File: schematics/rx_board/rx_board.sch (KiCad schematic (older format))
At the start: 15 parts, among them U1 SI4463-C2A-GM, X2 SMA

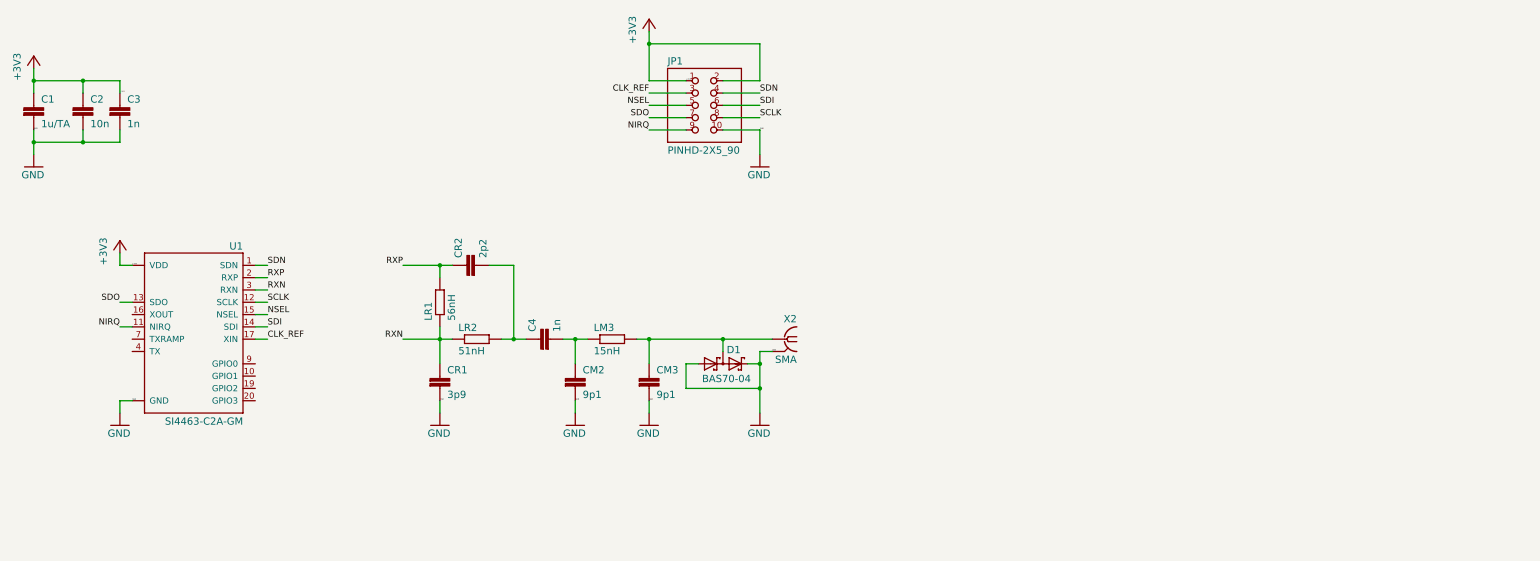
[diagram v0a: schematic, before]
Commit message: first complete design & routing
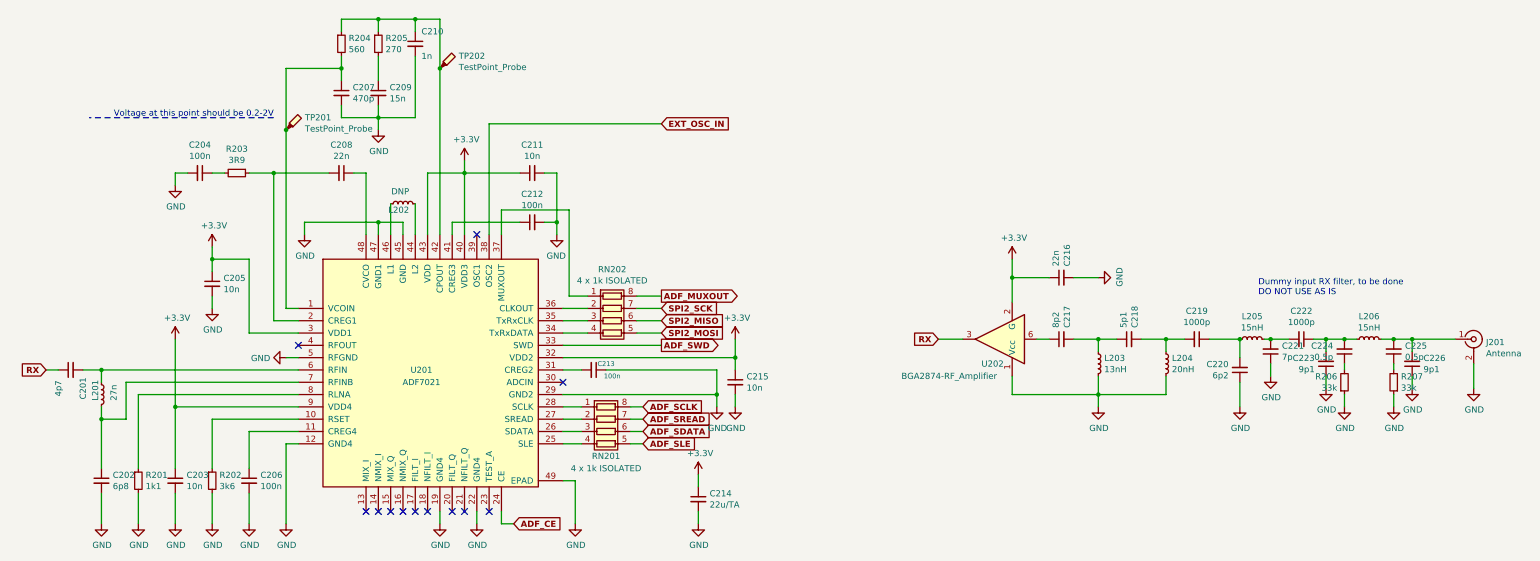
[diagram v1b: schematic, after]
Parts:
- removed C1: 1u/TA, rx_board:C1206, symbol rx_board-eagle-import:C-EUC1206
- removed C2: 10n, rx_board:C0805, symbol rx_board-eagle-import:C-EUC0805
- removed C3, C4: 1n, rx_board:C0805, symbol rx_board-eagle-import:C-EUC0805
- removed CM2, CM3: 9p1, rx_board:C0805, symbol rx_board-eagle-import:C-EUC0805
- removed CR1: 3p9, rx_board:C0805, symbol rx_board-eagle-import:C-EUC0805
- removed CR2: 2p2, rx_board:C0805, symbol rx_board-eagle-import:C-EUC0805
- removed D1: BAS70-04, rx_board:SOT23, symbol rx_board-eagle-import:BAS70-04
- removed JP1: PINHD-2X5_90, rx_board:2X05_90, symbol rx_board-eagle-import:PINHD-2X5_90
- removed LM3: 15nH, rx_board:R0805, symbol rx_board-eagle-import:R-EU_R0805
- removed LR1: 56nH, rx_board:R0805, symbol rx_board-eagle-import:R-EU_R0805
- removed LR2: 51nH, rx_board:R0805, symbol rx_board-eagle-import:R-EU_R0805
- removed U1: SI4463-C2A-GM, rx_board:QFN50P400X400X90-20N, symbol rx_board-eagle-import:SI4463-C2A-GM
- removed X2: SMA, rx_board:J502-ND-142-0701-871_876, symbol rx_board-eagle-import:SMA-142-0701-871_876
- added C201: 4p7, Capacitor_SMD:C_0603_1608Metric, symbol rx_board-rescue:C_Small-Device-Mainboard-rescue-rx_board-rescue
- added C202: 6p8, Capacitor_SMD:C_0603_1608Metric, symbol rx_board-rescue:C_Small-Device-Mainboard-rescue-rx_board-rescue
- added C203, C205, C211, C215: 10n, Capacitor_SMD:C_0603_1608Metric, symbol rx_board-rescue:C_Small-Device-Mainboard-rescue-rx_board-rescue
- added C204, C206, C212, C213: 100n, Capacitor_SMD:C_0603_1608Metric, symbol rx_board-rescue:C_Small-Device-Mainboard-rescue-rx_board-rescue
- added C207: 470p, Capacitor_SMD:C_0603_1608Metric, symbol rx_board-rescue:C_Small-Device-Mainboard-rescue-rx_board-rescue
- added C208, C216: 22n, Capacitor_SMD:C_0603_1608Metric, symbol rx_board-rescue:C_Small-Device-Mainboard-rescue-rx_board-rescue
- added C209: 15n, Capacitor_SMD:C_0603_1608Metric, symbol rx_board-rescue:C_Small-Device-Mainboard-rescue-rx_board-rescue
- added C210: 1n, Capacitor_SMD:C_0603_1608Metric, symbol rx_board-rescue:C_Small-Device-Mainboard-rescue-rx_board-rescue
- added C214: 22u/TA, Capacitor_Tantalum_SMD:CP_EIA-3216-18_Kemet-A, symbol rx_board-rescue:C_Small-device-Mainboard-rescue-rx_board-rescue
- added C217: 8p2, Capacitor_SMD:C_0603_1608Metric, symbol rx_board-rescue:C_Small-Device-Mainboard-rescue-rx_board-rescue
- added C218: 5p1, Capacitor_SMD:C_0603_1608Metric, symbol rx_board-rescue:C_Small-Device-Mainboard-rescue-rx_board-rescue
- added C219, C222: 1000p, Capacitor_SMD:C_0603_1608Metric, symbol rx_board-rescue:C_Small-device-Mainboard-rescue-rx_board-rescue
- added C220: 6p2, Capacitor_SMD:C_0603_1608Metric, symbol rx_board-rescue:C_Small-Device-Mainboard-rescue-rx_board-rescue
- added C221: 7p, Capacitor_SMD:C_0603_1608Metric, symbol rx_board-rescue:C_Small-Device-Mainboard-rescue-rx_board-rescue
- added C223, C226: 9p1, Capacitor_SMD:C_0603_1608Metric, symbol rx_board-rescue:C_Small-device-Mainboard-rescue-rx_board-rescue
- added C224, C225: 0.5p, Capacitor_SMD:C_0603_1608Metric, symbol rx_board-rescue:C_Small-Device-Mainboard-rescue-rx_board-rescue
- added J201: Antenna, Connector_Coaxial:SMA_Samtec_SMA-J-P-X-ST-EM1_EdgeMount, symbol rx_board-rescue:Conn_Coaxial-conn-Mainboard-rescue-rx_board-rescue
- added L201: 27n, Inductor_SMD:L_0603_1608Metric, symbol rx_board-rescue:L_Small-Device-Mainboard-rescue-rx_board-rescue
- added L202: DNP, Inductor_SMD:L_0603_1608Metric, symbol rx_board-rescue:L_Small-Device-Mainboard-rescue-rx_board-rescue
- added L203: 13nH, Inductor_SMD:L_0603_1608Metric, symbol Device:L_Small
- added L204: 20nH, Inductor_SMD:L_0603_1608Metric, symbol Device:L_Small
- added L205: 15nH, Inductor_SMD:L_0603_1608Metric, symbol rx_board-rescue:L_Small-Device-Mainboard-rescue-rx_board-rescue
- added L206: 15nH, Inductor_SMD:L_0603_1608Metric, symbol rx_board-rescue:L_Small-device-Mainboard-rescue-rx_board-rescue
- added R201: 1k1, Resistor_SMD:R_0603_1608Metric, symbol rx_board-rescue:R_Small-Device-Mainboard-rescue-rx_board-rescue
- added R202: 3k6, Resistor_SMD:R_0603_1608Metric, symbol rx_board-rescue:R_Small-Device-Mainboard-rescue-rx_board-rescue
- added R203: 3R9, Resistor_SMD:R_0603_1608Metric, symbol rx_board-rescue:R_Small-Device-Mainboard-rescue-rx_board-rescue
- added R204: 560, Resistor_SMD:R_0603_1608Metric, symbol rx_board-rescue:R_Small-Device-Mainboard-rescue-rx_board-rescue
- added R205: 270, Resistor_SMD:R_0603_1608Metric, symbol rx_board-rescue:R_Small-Device-Mainboard-rescue-rx_board-rescue
- added R206, R207: 33k, Resistor_SMD:R_0603_1608Metric, symbol rx_board-rescue:R_Small-Device-Mainboard-rescue-rx_board-rescue
- added RN201, RN202: 4 x 1k ISOLATED, Resistor_SMD:R_Array_Concave_4x0603, symbol Device:R_Pack04
- added TP201, TP202: TestPoint_Probe, TestPoint:TestPoint_Pad_D1.0mm, symbol rx_board-rescue:TestPoint_Probe-Connector-Mainboard-rescue-rx_board-rescue
- added U201: ADF7021, Package_CSP:LFCSP-48-1EP_7x7mm_P0.5mm_EP4.1x4.1mm_ThermalVias, symbol rx_board-rescue:ADF7021-adf7021-rx_board-rescue
- added U202: BGA2874-RF_Amplifier, Package_TO_SOT_SMD:SOT-363_SC-70-6, symbol bga2874-rf_amplifier:BGA2874-RF_Amplifier
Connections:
- net +3V3: now also C203.1, C205.1, C211.1, C214.1, C215.1, C216.1, U201.3 (VDD1), U201.32 (VDD2), U201.40 (VDD3), U201.43 (VDD), U201.9 (VDD4), U202.2 (G), U202.4 (G), U202.5 (G)
- net GND: now also C202.2, C203.2, C204.2, C205.2, C206.2, C207.2, C209.2, C210.2, C211.2, C212.2, C213.1, C214.2, C215.2, C216.2, C220.1, C221.1, C223.1, C226.1, J201.2 (Ext), L203.2, L204.2, R201.2, R202.2, R206.1, R207.1, U201.12 (GND4), U201.19 (GND4), U201.22 (GND4), U201.29 (GND2), U201.45 (GND), U201.47 (GND1), U201.49 (EPAD), U201.5 (RFGND), U202.1 (Vcc)
- new net: C219.1, C220.2, L205.1
- new net: C218.2, C219.2, L204.1
- new net: C221.2, C222.2, L205.2
- new net: C225.2, C226.2, J201.1 (In), L206.2
- new net: C222.1, C223.2, C224.2, L206.1
- new net: C224.1, R206.2
- new net: C225.1, R207.2
- new net: C207.1, R204.2, TP201.1, U201.1 (VCOIN)
- new net: R202.1, U201.10 (RSET)
- new net: C206.1, U201.11 (CREG4)
- new net: C208.2, R203.1, U201.2 (CREG1)
- new net: RN201.4 (R4.1), U201.25 (SLE)
- new net: RN201.3 (R3.1), U201.26 (SDATA)
- new net: RN201.2 (R2.1), U201.27 (SREAD)
- new net: RN201.1 (R1.1), U201.28 (SCLK)
- new net: C213.2, U201.31 (CREG2)
- new net: RN202.4 (R4.1), U201.34 (TxRxDATA)
- new net: RN202.3 (R3.1), U201.35 (TxRxCLK)
- new net: RN202.2 (R2.1), U201.36 (CLKOUT)
- new net: RN202.1 (R1.1), U201.37 (MUXOUT)
- new net: C212.1, U201.41 (CREG3)
- new net: C210.1, R204.1, R205.1, TP202.1, U201.42 (CPOUT)
- new net: L202.2, U201.44 (L2)
- new net: L202.1, U201.46 (L1)
- new net: C208.1, U201.48 (CVCO)
- new net: C201.2, L201.1, U201.6 (RFIN)
- new net: C202.1, L201.2, U201.7 (RFINB)
- new net: R201.1, U201.8 (RLNA)
- new net: C204.1, R203.2
- new net: C209.1, R205.2
- new net: C217.2, C218.1, L203.1
- new net: C217.1, U202.6
- new net ADF_CE: U201.24 (CE)
- new net ADF_MUXOUT: RN202.8 (R1.2)
- new net ADF_SCLK: RN201.8 (R1.2)
- new net ADF_SDATA: RN201.6 (R3.2)
- new net ADF_SLE: RN201.5 (R4.2)
- new net ADF_SREAD: RN201.7 (R2.2)
- new net ADF_SWD: U201.33 (SWD)
- new net EXT_OSC_IN: U201.38 (OSC2)
- new net RX: C201.1, U202.3
- new net SPI2_MISO: RN202.6 (R3.2)
- new net SPI2_MOSI: RN202.5 (R4.2)
- new net SPI2_SCK: RN202.7 (R2.2)
- no-connect marks 0 -> 12
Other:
- note added: "Dummy input RX filter, to be done\nDO NOT USE AS IS"
- note added: "Voltage at this point should be 0.2-2V"
